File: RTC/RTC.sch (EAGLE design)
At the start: 8 parts, among them IC1 DS3231/SO

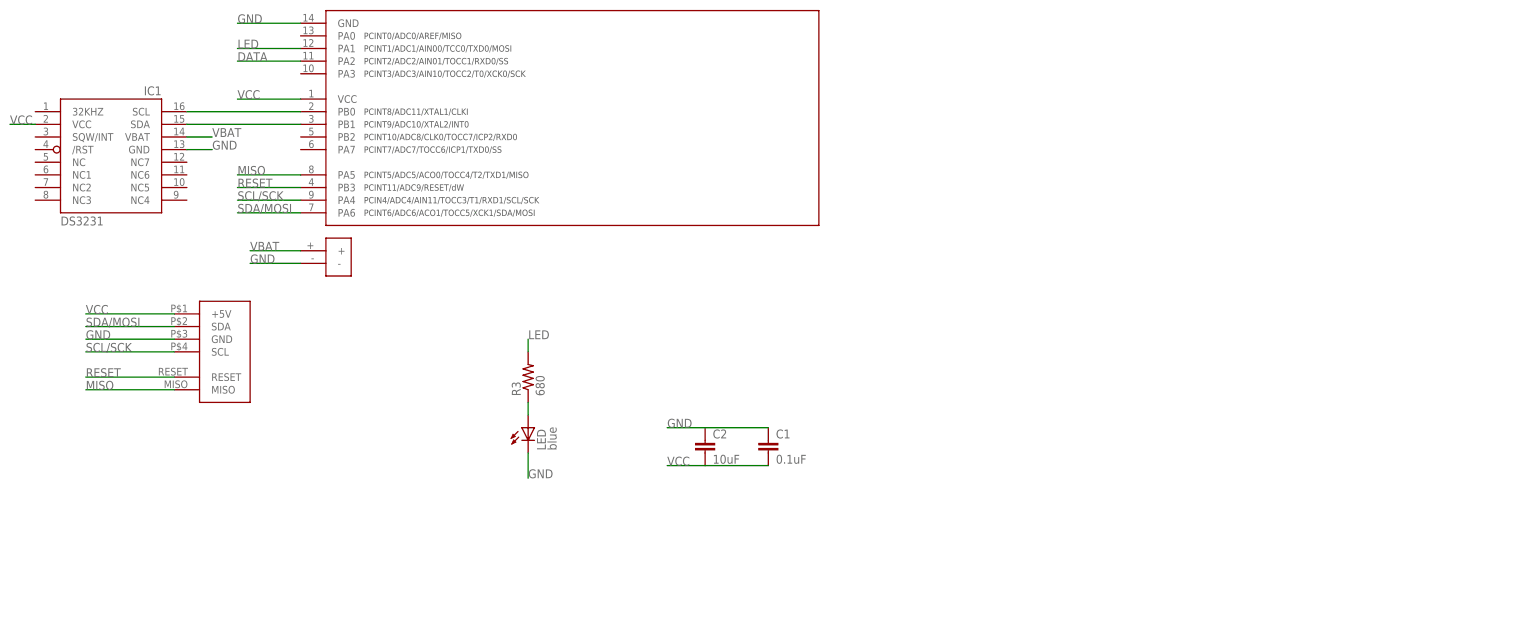
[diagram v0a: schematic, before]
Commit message: Latest version of schematics and boards
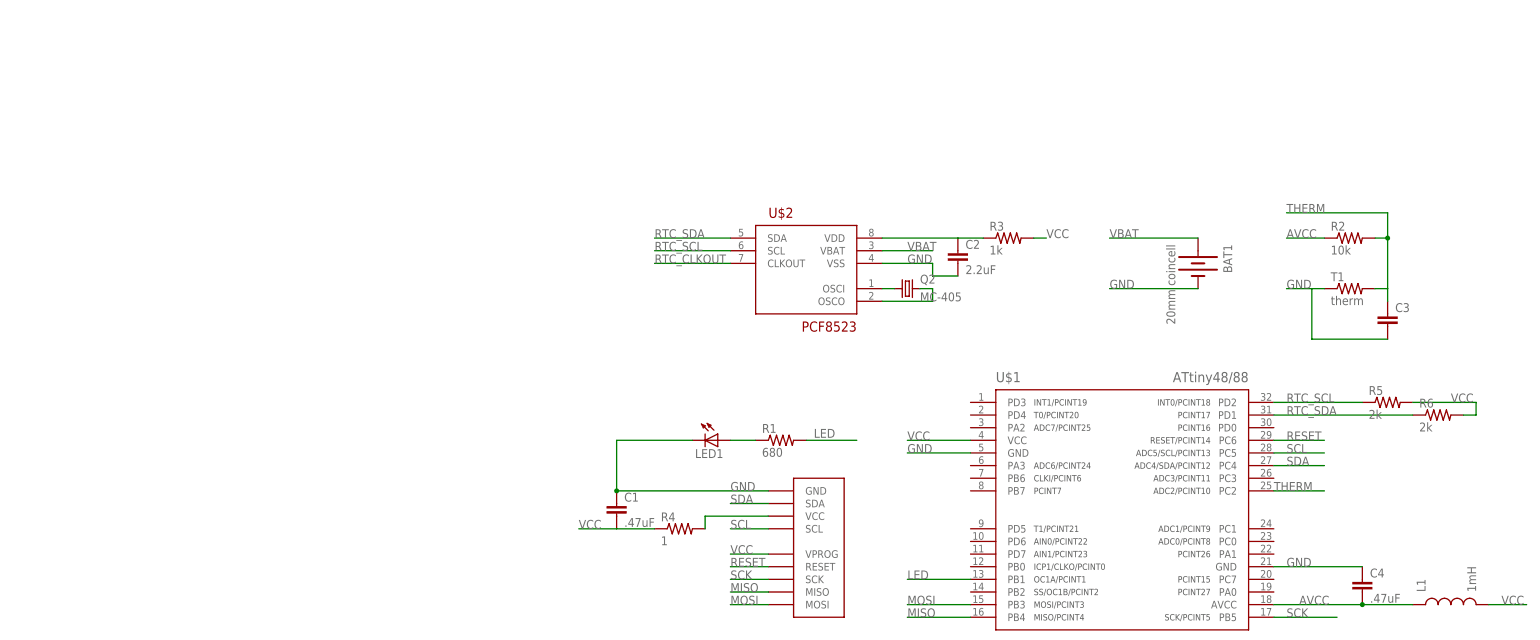
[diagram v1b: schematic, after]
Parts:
- removed IC1: DS3231/SO, adafruit:DS3231/SO
- removed LED: blue, led:LEDCHIPLED_1206
- removed U$3: TINY841, IntegerLabs:TINY841
- added BAT1: 20mm coincell, SparkFun-Electromechanical:BATTERY20MM_4LEGS
- added C3: (no value), SparkFun-Capacitors:CAP0805
- added C4: .47uF, SparkFun-Capacitors:CAP0805
- added L1: 1mH, SparkFun-Passives:INDUCTOR1007
- added LED1: (no value), adafruit:LEDCHIP-LED0805
- added Q2: MC-405, crystal:MC-405
- added R1: 680, SparkFun-Passives:RESISTOR0805-RES
- added R2: 10k, SparkFun-Passives:RESISTOR0805-RES
- added R4: 1, SparkFun-Resistors:RESISTOR0805-RES
- added R5, R6: 2k, SparkFun-Resistors:RESISTOR0805-RES
- added T1: therm, SparkFun-Passives:RESISTOR0805-RES
- added U$1: ATTINY48/88-TQFP, IntegerLabs:ATTINY48/88-TQFP
- C1: value 0.1uF -> .47uF
- C2: value 10uF -> 2.2uF; device SparkFun-Capacitors:CAP0805 -> SparkFun-Passives:CAP0805
- R3: value 680 -> 1k
- U$2: value BATTERY -> PCF8523; device IntegerLabs:BATTERY -> IntegerLabs:PCF8523
- U$4: value FOOTPRINT -> FOOTPRINTFOOTPRINT-2; device IntegerLabs:FOOTPRINT -> IntegerLabs:FOOTPRINTFOOTPRINT-2
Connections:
- removed net DATA: U$3.PA2
- removed net SCL/SCK: U$3.PA4, U$4.SCL
- removed net SDA/MOSI: U$3.PA6, U$4.SDA
- new net AVCC: C4.2, L1.1, R2.1, U$1.AVCC
- new net MOSI: U$1.PB3, U$4.MOSI
- new net N$7: Q2.1, U$2.OSCI
- new net N$8: Q2.2, U$2.OSCO
- new net RTC_CLKOUT: U$2.CLKOUT
- new net RTC_SCL: R5.1, U$1.PD2, U$2.SCL
- new net RTC_SDA: R6.1, U$1.PD1, U$2.SDA
- new net SCK: U$1.PB5, U$4.SCK
- new net SCL: U$1.PC5, U$4.SCL
- new net SDA: U$1.PC4, U$4.SDA
- new net THERM: C3.1, R2.2, T1.2, U$1.PC2
- net GND: now also BAT1.-, C2.2, C3.2, C4.1, LED1.C, T1.1, U$1.GND, U$1.GND@1, U$2.VSS; no longer C2.1, IC1.GND, LED.C, U$2.-, U$3.GND
- net LED: now also R1.2, U$1.PB1; no longer R3.2, U$3.PA1
- net MISO: now also U$1.PB4; no longer U$3.PA5
- net N$2: now also R4.2, U$4.VCC; no longer IC1.SCL, U$3.PB0
- net N$3: now also C2.1, R3.1, U$2.VDD; no longer IC1.SDA, U$3.PB1
- net N$5: now also LED1.A, R1.1; no longer LED.A, R3.1
- net RESET: now also U$1.PC6; no longer U$3.PB3
- net VBAT: now also BAT1.+, U$2.VBAT; no longer IC1.VBAT, U$2.+
- net VCC: now also L1.2, R3.2, R4.1, R5.2, R6.2, U$1.VCC, U$4.VPROG; no longer C2.2, IC1.VCC, U$3.VCC, U$4.+5V
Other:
- moved on the sheet: C1, C2, R3
